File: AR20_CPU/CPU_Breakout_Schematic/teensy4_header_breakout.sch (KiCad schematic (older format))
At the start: 11 parts, among them J3 Micro_SD_Card, SW1 SW_SPST, U1 Teensy_pins, U2 MCP2551-I-SN

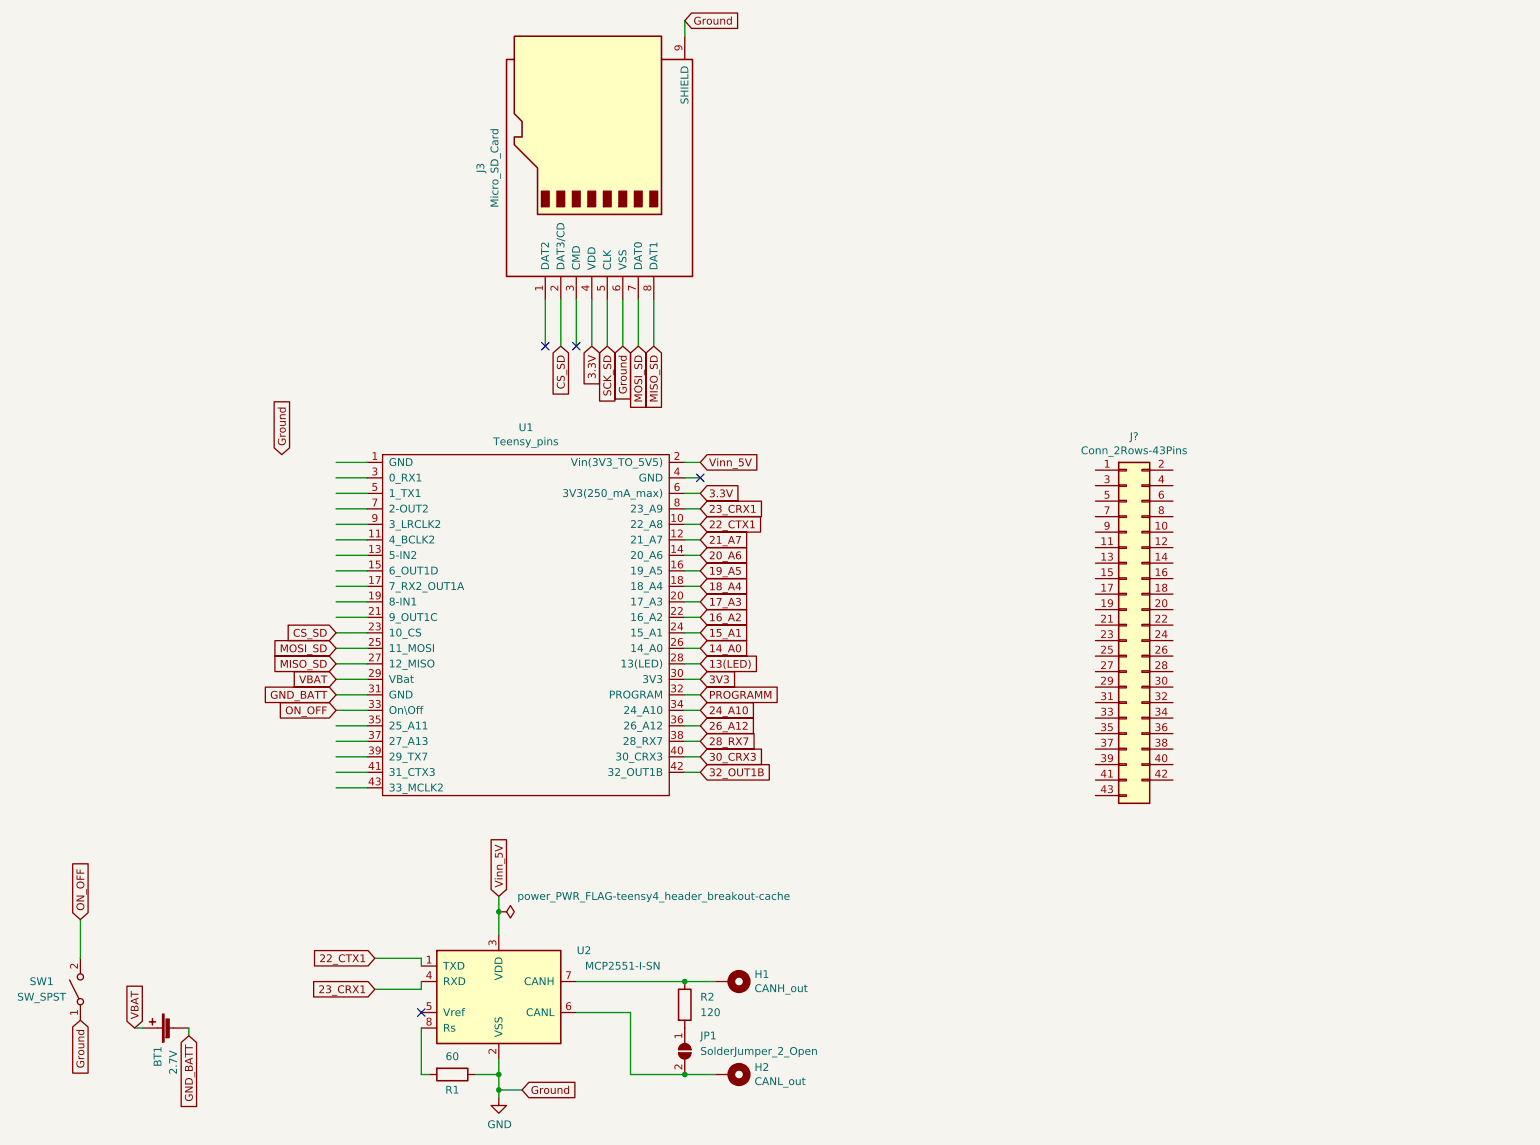
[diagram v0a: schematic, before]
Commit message: FOOTPRINT IS DONE
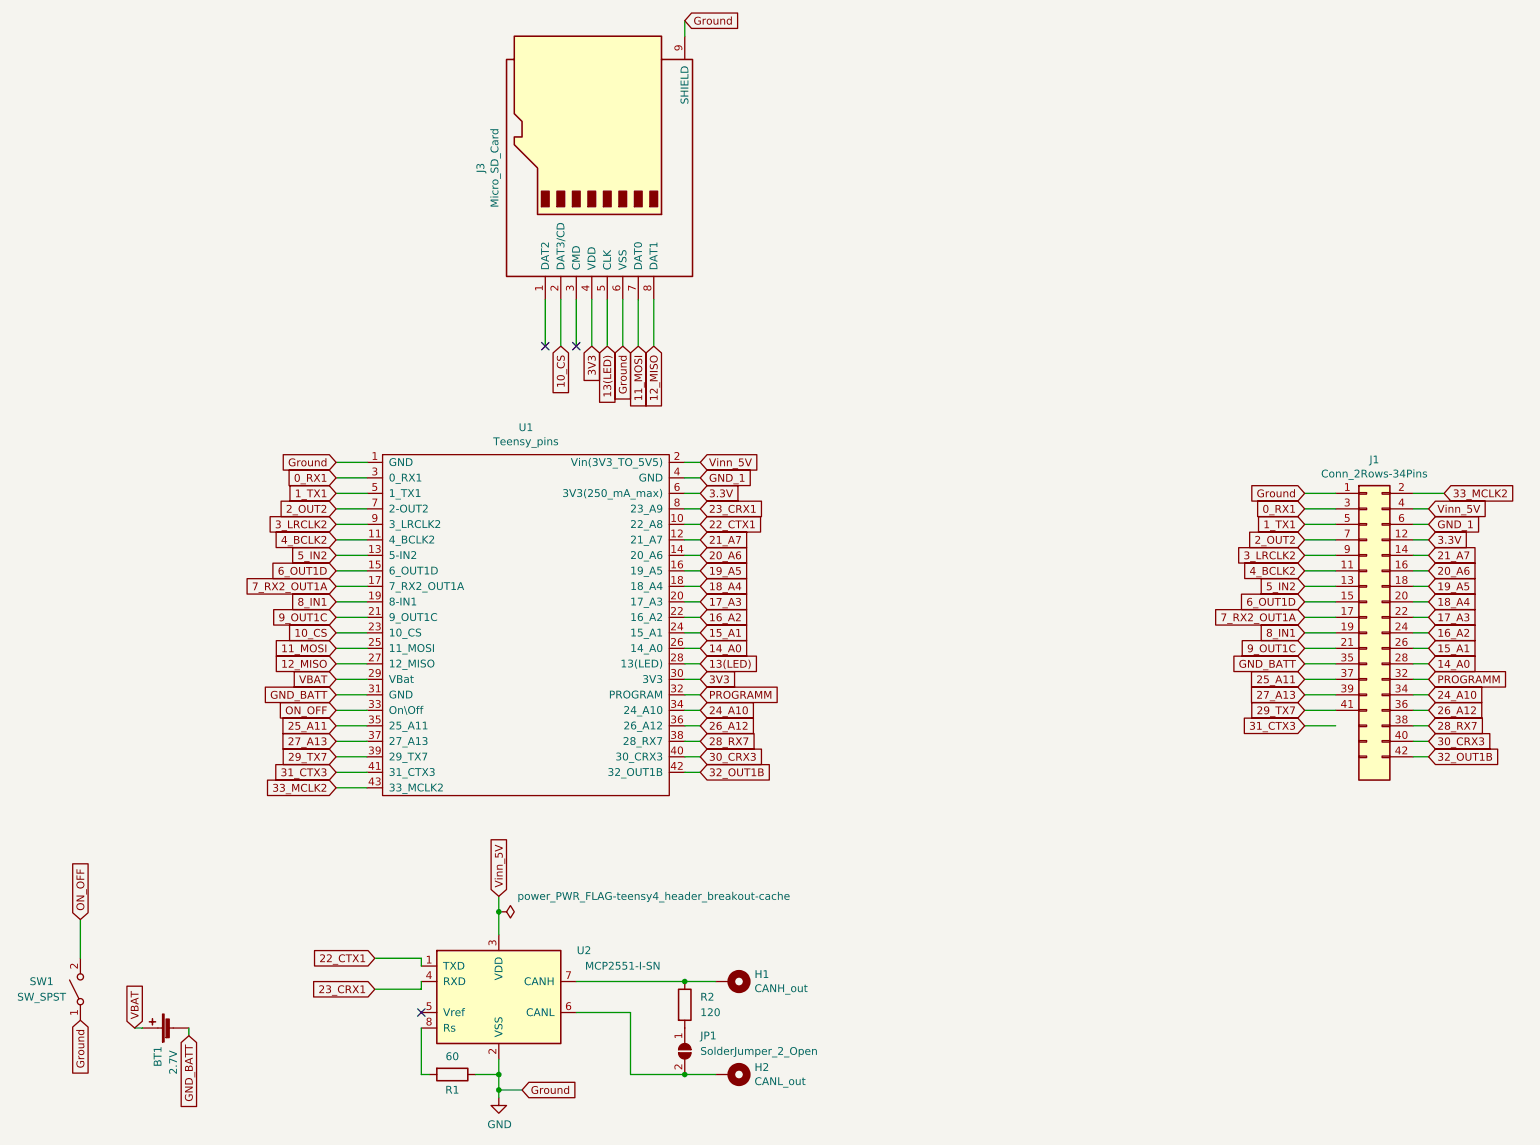
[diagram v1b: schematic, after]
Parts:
- removed J?: Conn_2Rows-43Pins, symbol Connector_Generic:Conn_2Rows-43Pins
- added J1: Conn_2Rows-34Pins, Teensy_Footprint_Library:PINS_IO_TEENSY, symbol BreakoutBoardTeensy:Conn_2Rows-34Pins
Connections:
- net labels added: 0_RX1, 10_CS, 11_MOSI, 12_MISO, 1_TX1, 25_A11, 27_A13, 29_TX7, 2_OUT2, 31_CTX3, 33_MCLK2, 3_LRCLK2, 4_BCLK2, 5_IN2, 6_OUT1D, 7_RX2_OUT1A, 8_IN1, 9_OUT1C, GND_1
- net labels removed: CS_SD, MISO_SD, MOSI_SD, SCK_SD
- wire segments 74 -> 108
- no-connect marks 4 -> 3
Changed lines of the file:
@@
 Text GLabel 2850 6850 0    50   Input ~ 0
 23_CRX1
-Text GLabel 4950 3850 2    50   Input ~ 0
-22_CTX1
-Text GLabel 4950 3750 2    50   Input ~ 0
-23_CRX1
 Text GLabel 3650 6250 1    50   Input ~ 0
 Vinn_5V
-Text GLabel 4950 3450 2    50   Input ~ 0
-Vinn_5V
 $Comp
 L power:GND #PWR0101
@@
 Text GLabel 4450 2700 3    50   Input ~ 0
 Ground
-Text GLabel 2250 3400 1    50   Input ~ 0
+Text GLabel 2600 3450 0    50   Input ~ 0
 Ground
 $Comp
@@
 VBAT
 Text GLabel 2600 4750 0    50   Input ~ 0
-MISO_SD
-Text GLabel 2600 4650 0    50   Input ~ 0
-MOSI_SD
-Text GLabel 2600 4550 0    50   Input ~ 0
-CS_SD
-Text GLabel 4950 4750 2    50   Input ~ 0
-13(LED)
-Text GLabel 4350 2700 3    50   Input ~ 0
-SCK_SD
-Text GLabel 4650 2700 3    50   Input ~ 0
-MISO_SD
-Text GLabel 4550 2700 3    50   Input ~ 0
-MOSI_SD
-Text GLabel 4050 2700 3    50   Input ~ 0
-CS_SD
+12_MISO
 $Bitmap
 Pos 1650 1500
@@
 EndData
 $EndBitmap
-Wire Wire Line
-	4850 3450 4950 3450
-Wire Wire Line
-	4850 3550 4950 3550
-Wire Wire Line
-	4850 3750 4950 3750
-Wire Wire Line
-	4850 3850 4950 3850
 Connection ~ 3650 6350
 Wire Wire Line
@@
 NoConn ~ 3950 2700
 NoConn ~ 4150 2700
-NoConn ~ 4950 3550
 Text GLabel 4850 600  2    50   Input ~ 0
 Ground
 Wire Wire Line
 	4850 700  4850 600
-Text GLabel 4950 3650 2    50   Input ~ 0
-3.3V
-Text GLabel 4250 2700 3    50   Input ~ 0
-3.3V
 Wire Wire Line
 	4250 2400 4250 2700
-$Comp
-L BreakoutBoardTeensy:Teensy_pins U1
-U 1 1 5DD8E484
-P 3250 4150
-F 0 "U1" H 3825 5075 50  0000 C CNN
-F 1 "Teensy_pins" H 3825 4984 50  0000 C CNN
-F 2 "Teensy_Footprint_Library:Teensy_40_footprint" H 4550 4150 50  0001 C CNN
-F 3 "" H 4550 4150 50  0001 C CNN
-	1    3250 4150
-	1    0    0    -1
-$EndComp
 Wire Wire Line
 	2800 4850 2600 4850
@@
 	0    1    1    0
 $EndComp
-$Comp
-L Connector_Generic:Conn_2Rows-43Pins J?
-U 1 1 5DDC3E02
-P 7700 4500
-F 0 "J?" H 7750 5717 50  0000 C CNN
-F 1 "Conn_2Rows-43Pins" H 7750 5626 50  0000 C CNN
-F 2 "" H 7700 4500 50  0001 C CNN
-F 3 "~" H 7700 4500 50  0001 C CNN
-	1    7700 4500
-	1    0    0    -1
-$EndComp
 Wire Wire Line
 	2600 4750 2800 4750
@@
 Wire Wire Line
 	2800 3450 2600 3450
+Text GLabel 2600 3550 0    50   Input ~ 0
+0_RX1
+Text GLabel 2600 3650 0    50   Input ~ 0
+1_TX1
+Text GLabel 2600 3750 0    50   Input ~ 0
+2_OUT2
+Text GLabel 2600 3850 0    50   Input ~ 0
+3_LRCLK2
+Text GLabel 2600 3950 0    50   Input ~ 0
+4_BCLK2
+Text GLabel 2600 4050 0    50   Input ~ 0
+5_IN2
+Text GLabel 2600 4150 0    50   Input ~ 0
+6_OUT1D
+Text GLabel 2600 4250 0    50   Input ~ 0
+7_RX2_OUT1A
+Text GLabel 2600 4350 0    50   Input ~ 0
+8_IN1
+Text GLabel 2600 4450 0    50   Input ~ 0
+9_OUT1C
+Text GLabel 2600 5150 0    50   Input ~ 0
+25_A11
+Text GLabel 2600 5250 0    50   Input ~ 0
+27_A13
+Text GLabel 2600 5350 0    50   Input ~ 0
+29_TX7
+Text GLabel 2600 5450 0    50   Input ~ 0
+31_CTX3
+Text GLabel 2600 5550 0    50   Input ~ 0
+33_MCLK2
+Text GLabel 2600 4550 0    50   Input ~ 0
+10_CS
+Text GLabel 2600 4650 0    50   Input ~ 0
+11_MOSI
+Text GLabel 8850 4750 0    50   Input ~ 0
+GND_BATT
+Text GLabel 8850 3650 0    50   Input ~ 0
+Ground
 Wire Wire Line
-	4850 3950 4950 3950
+	9050 4750 8850 4750
 Wire Wire Line
-	4850 4050 4950 4050
+	9050 4850 8850 4850
 Wire Wire Line
-	4850 4150 4950 4150
+	9050 4950 8850 4950
 Wire Wire Line
-	4850 4250 4950 4250
+	9050 5050 8850 5050
 Wire Wire Line
-	4850 4350 4950 4350
+	9050 5150 8850 5150
 Wire Wire Line
-	4850 4450 4950 4450
+	9550 3650 9750 3650
 Wire Wire Line
-	4850 4550 4950 4550
+	9050 4650 8850 4650
 Wire Wire Line
-	4850 4650 4950 4650
+	9050 4550 8850 4550
 Wire Wire Line
-	4850 4850 4950 4850
+	9050 4450 8850 4450
 Wire Wire Line
-	4850 4950 4950 4950
+	9050 4350 8850 4350
 Wire Wire Line
-	4850 5050 4950 5050
+	9050 4250 8850 4250
 Wire Wire Line
-	4850 5150 4950 5150
+	9050 4150 8850 4150
 Wire Wire Line
-	4850 5250 4950 5250
+	9050 4050 8850 4050
 Wire Wire Line
-	4850 5350 4950 5350
+	9050 3950 8850 3950
 Wire Wire Line
-	4850 5450 4950 5450
+	9050 3850 8850 3850
 Wire Wire Line
-	4950 3650 4850 3650
-Text GLabel 4950 3950 2    50   Input ~ 0
-21_A7
-Text GLabel 4950 4050 2    50   Input ~ 0
-20_A6
-Text GLabel 4950 4150 2    50   Input ~ 0
-19_A5
-Text GLabel 4950 4250 2    50   Input ~ 0
-18_A4
-Text GLabel 4950 4350 2    50   Input ~ 0
-17_A3
-Text GLabel 4950 4450 2    50   Input ~ 0
-16_A2
-Text GLabel 4950 4550 2    50   Input ~ 0
-15_A1
-Text GLabel 4950 4650 2    50   Input ~ 0
-14_A0
-Text GLabel 4950 4850 2    50   Input ~ 0
-3V3
-Text GLabel 4950 4950 2    50   Input ~ 0
-PROGRAMM
-Text GLabel 4950 5050 2    50   Input ~ 0
-24_A10
-Text GLabel 4950 5150 2    50   Input ~ 0
-26_A12
-Text GLabel 4950 5250 2    50   Input ~ 0
-28_RX7
+	9050 3750 8850 3750
+Wire Wire Line
+	9050 3650 8850 3650
+Text GLabel 8850 3750 0    50   Input ~ 0
+0_RX1
+Text GLabel 8850 3850 0    50   Input ~ 0
+1_TX1
+Text GLabel 8850 3950 0    50   Input ~ 0
+2_OUT2
+Text GLabel 8850 4050 0    50   Input ~ 0
+3_LRCLK2
+Text GLabel 8850 4150 0    50   Input ~ 0
+4_BCLK2
+Text GLabel 8850 4250 0    50   Input ~ 0
+5_IN2
+Text GLabel 8850 4350 0    50   Input ~ 0
+6_OUT1D
+Text GLabel 8850 4450 0    50   Input ~ 0
+7_RX2_OUT1A
+Text GLabel 8850 4550 0    50   Input ~ 0
+8_IN1
+Text GLabel 8850 4650 0    50   Input ~ 0
+9_OUT1C
+Text GLabel 8850 4850 0    50   Input ~ 0
+25_A11
+Text GLabel 8850 4950 0    50   Input ~ 0
+27_A13
+Text GLabel 8850 5050 0    50   Input ~ 0
+29_TX7
+Text GLabel 8850 5150 0    50   Input ~ 0
+31_CTX3
+Text GLabel 9750 3650 2    50   Input ~ 0
+33_MCLK2
+Wire Wire Line
+	4950 4750 4850 4750
+Text GLabel 4950 5450 2    50   Input ~ 0
+32_OUT1B
 Text GLabel 4950 5350 2    50   Input ~ 0
 30_CRX3
-Text GLabel 4950 5450 2    50   Input ~ 0
+Text GLabel 4950 5250 2    50   Input ~ 0
+28_RX7
+Text GLabel 4950 5150 2    50   Input ~ 0
+26_A12
+Text GLabel 4950 5050 2    50   Input ~ 0
+24_A10
+Text GLabel 4950 4950 2    50   Input ~ 0
+PROGRAMM
+Text GLabel 4950 4850 2    50   Input ~ 0
+3V3
+Text GLabel 4950 4650 2    50   Input ~ 0
+14_A0
+Text GLabel 4950 4550 2    50   Input ~ 0
+15_A1
+Text GLabel 4950 4450 2    50   Input ~ 0
+16_A2
+Text GLabel 4950 4350 2    50   Input ~ 0
+17_A3
+Text GLabel 4950 4250 2    50   Input ~ 0
+18_A4
+Text GLabel 4950 4150 2    50   Input ~ 0
+19_A5
+Text GLabel 4950 4050 2    50   Input ~ 0
+20_A6
+Text GLabel 4950 3950 2    50   Input ~ 0
+21_A7
+Wire Wire Line
+	4950 3650 4850 3650
+Wire Wire Line
+	4850 5450 4950 5450
+Wire Wire Line
+	4850 5350 4950 5350
+Wire Wire Line
+	4850 5250 4950 5250
+Wire Wire Line
+	4850 5150 4950 5150
+Wire Wire Line
+	4850 5050 4950 5050
+Wire Wire Line
+	4850 4950 4950 4950
+Wire Wire Line
+	4850 4850 4950 4850
+Wire Wire Line
+	4850 4650 4950 4650
+Wire Wire Line
+	4850 4550 4950 4550
+Wire Wire Line
+	4850 4450 4950 4450
+Wire Wire Line
+	4850 4350 4950 4350
+Wire Wire Line
+	4850 4250 4950 4250
+Wire Wire Line
+	4850 4150 4950 4150
+Wire Wire Line
+	4850 4050 4950 4050
+Wire Wire Line
+	4850 3950 4950 3950
+Text GLabel 4950 3650 2    50   Input ~ 0
+3.3V
+Wire Wire Line
+	4850 3850 4950 3850
+Wire Wire Line
+	4850 3750 4950 3750
+Wire Wire Line
+	4850 3550 4950 3550
+Wire Wire Line
+	4850 3450 4950 3450
+Text GLabel 4950 4750 2    50   Input ~ 0
+13(LED)
+Text GLabel 4950 3450 2    50   Input ~ 0
+Vinn_5V
+Text GLabel 4950 3750 2    50   Input ~ 0
+23_CRX1
+Text GLabel 4950 3850 2    50   Input ~ 0
+22_CTX1
+Text GLabel 9650 5350 2    50   Input ~ 0
 32_OUT1B
+Text GLabel 9650 5250 2    50   Input ~ 0
+30_CRX3
+Text GLabel 9650 5150 2    50   Input ~ 0
+28_RX7
+Text GLabel 9650 5050 2    50   Input ~ 0
+26_A12
+Text GLabel 9650 4950 2    50   Input ~ 0
+24_A10
+Text GLabel 9650 4850 2    50   Input ~ 0
+PROGRAMM
+Text GLabel 9650 4750 2    50   Input ~ 0
+14_A0
+Text GLabel 9650 4650 2    50   Input ~ 0
+15_A1
+Text GLabel 9650 4550 2    50   Input ~ 0
+16_A2
+Text GLabel 9650 4450 2    50   Input ~ 0
+17_A3
+Text GLabel 9650 4350 2    50   Input ~ 0
+18_A4
+Text GLabel 9650 4250 2    50   Input ~ 0
+19_A5
+Text GLabel 9650 4150 2    50   Input ~ 0
+20_A6
+Text GLabel 9650 4050 2    50   Input ~ 0
+21_A7
 Wire Wire Line
-	4950 4750 4850 4750
+	9550 5350 9650 5350
+Wire Wire Line
+	9550 5250 9650 5250
+Wire Wire Line
+	9550 5150 9650 5150
+Wire Wire Line
+	9550 5050 9650 5050
+Wire Wire Line
+	9550 4950 9650 4950
+Wire Wire Line
+	9550 4850 9650 4850
+Wire Wire Line
+	9550 4750 9650 4750
+Wire Wire Line
+	9550 4650 9650 4650
+Wire Wire Line
+	9550 4550 9650 4550
+Wire Wire Line
+	9550 4450 9650 4450
+Wire Wire Line
+	9550 4350 9650 4350
+Wire Wire Line
+	9550 4250 9650 4250
+Wire Wire Line
+	9550 4150 9650 4150
+Wire Wire Line
+	9550 4050 9650 4050
+Wire Wire Line
+	9550 3950 9650 3950
+Wire Wire Line
+	9550 3850 9650 3850
+Wire Wire Line
+	9550 3750 9650 3750
+Text GLabel 9650 3750 2    50   Input ~ 0
+Vinn_5V
+Text GLabel 4650 2700 3    50   Input ~ 0
+12_MISO
+Text GLabel 4550 2700 3    50   Input ~ 0
+11_MOSI
+Text GLabel 4050 2700 3    50   Input ~ 0
+10_CS
+Text GLabel 4350 2700 3    50   Input ~ 0
+13(LED)
+Text GLabel 9650 3850 2    50   Input ~ 0
+GND_1
+Text GLabel 4950 3550 2    50   Input ~ 0
+GND_1
+Text GLabel 4250 2700 3    50   Input ~ 0
+3V3
+Text GLabel 9650 3950 2    50   Input ~ 0
+3.3V
+$Comp
+L BreakoutBoardTeensy:Conn_2Rows-34Pins J1
+U 1 1 5DE58733
+P 9250 4550
+F 0 "J1" H 9300 5667 50  0000 C CNN
+F 1 "Conn_2Rows-34Pins" H 9300 5576 50  0000 C CNN
+F 2 "Teensy_Footprint_Library:PINS_IO_TEENSY" H 9250 4550 50  0001 C CNN
+F 3 "~" H 9250 4550 50  0001 C CNN
+	1    9250 4550
+	1    0    0    -1
+$EndComp
+$Comp
+L BreakoutBoardTeensy:Teensy_pins U1
+U 1 1 5DE5DBF9
+P 3250 4150
+F 0 "U1" H 3825 5075 50  0000 C CNN
+F 1 "Teensy_pins" H 3825 4984 50  0000 C CNN
+F 2 "Teensy_Footprint_Library:Teensy_40_footprint" H 4550 4150 50  0001 C CNN
+F 3 "" H 4550 4150 50  0001 C CNN
+	1    3250 4150
+	1    0    0    -1
+$EndComp
 $EndSCHEMATC

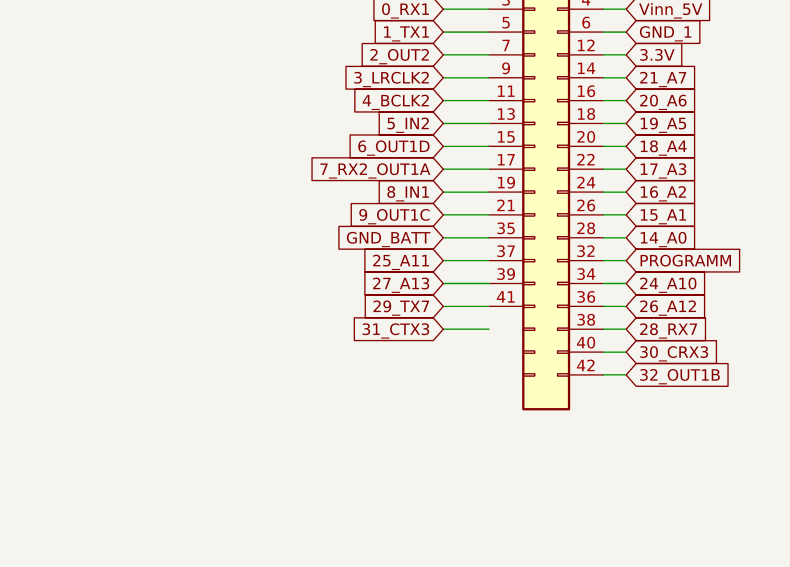
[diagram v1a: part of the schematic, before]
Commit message: initial traces is done
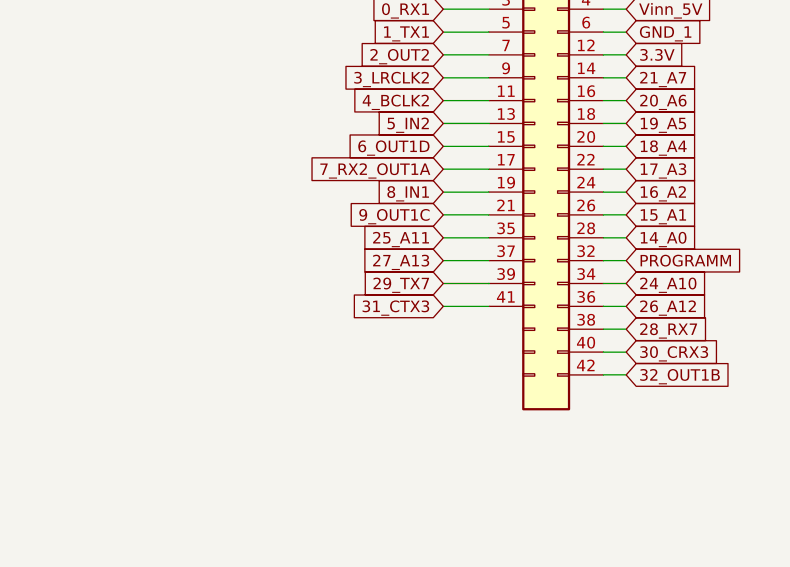
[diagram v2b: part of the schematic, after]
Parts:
- BT1: footprint Battery:BatteryHolder_Keystone_103_1x20mm -> Battery:BatteryHolder_Keystone_3034_1x20mm
- H1, H2: footprint TestPoint:TestPoint_THTPad_D1.0mm_Drill0.5mm -> TestPoint:TestPoint_THTPad_D1.5mm_Drill0.7mm
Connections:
- net 25_A11: now also J1.35 (Pin_35); no longer J1.37 (Pin_37)
- net 27_A13: now also J1.37 (Pin_37); no longer J1.39 (Pin_39)
- net 29_TX7: now also J1.39 (Pin_39); no longer J1.41 (Pin_41)
- net 31_CTX3: now also J1.41 (Pin_41)
- net GND_BATT: no longer J1.35 (Pin_35)
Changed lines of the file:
@@
 F 0 "BT1" H 1300 7200 50  0000 L CNN
 F 1 "2.7V " H 1250 7100 50  0000 L CNN
-F 2 "Battery:BatteryHolder_Keystone_103_1x20mm" V 1550 7160 50  0001 C CNN
+F 2 "Battery:BatteryHolder_Keystone_3034_1x20mm" V 1550 7160 50  0001 C CNN
 F 3 "~" V 1550 7160 50  0001 C CNN
 	1    1550 7100
@@
 F 0 "H2" V 5104 7550 50  0000 L CNN
 F 1 "CANL_out" V 5195 7550 50  0000 L CNN
-F 2 "TestPoint:TestPoint_THTPad_D1.0mm_Drill0.5mm" H 5150 7400 50  0001 C CNN
+F 2 "TestPoint:TestPoint_THTPad_D1.5mm_Drill0.7mm" H 5150 7400 50  0001 C CNN
 F 3 "~" H 5150 7400 50  0001 C CNN
 	1    5150 7400
@@
 F 0 "H1" V 5104 6950 50  0000 L CNN
 F 1 "CANH_out" V 5195 6950 50  0000 L CNN
-F 2 "TestPoint:TestPoint_THTPad_D1.0mm_Drill0.5mm" H 5150 6800 50  0001 C CNN
+F 2 "TestPoint:TestPoint_THTPad_D1.5mm_Drill0.7mm" H 5150 6800 50  0001 C CNN
 F 3 "~" H 5150 6800 50  0001 C CNN
 	1    5150 6800
@@
 Text GLabel 2600 4650 0    50   Input ~ 0
 11_MOSI
-Text GLabel 8850 4750 0    50   Input ~ 0
-GND_BATT
 Text GLabel 8850 3650 0    50   Input ~ 0
 Ground
@@
 	9050 5050 8850 5050
 Wire Wire Line
-	9050 5150 8850 5150
-Wire Wire Line
 	9550 3650 9750 3650
 Wire Wire Line
@@
 Text GLabel 8850 4650 0    50   Input ~ 0
 9_OUT1C
-Text GLabel 8850 4850 0    50   Input ~ 0
+Text GLabel 8850 4750 0    50   Input ~ 0
 25_A11
-Text GLabel 8850 4950 0    50   Input ~ 0
+Text GLabel 8850 4850 0    50   Input ~ 0
 27_A13
-Text GLabel 8850 5050 0    50   Input ~ 0
+Text GLabel 8850 4950 0    50   Input ~ 0
 29_TX7
-Text GLabel 8850 5150 0    50   Input ~ 0
+Text GLabel 8850 5050 0    50   Input ~ 0
 31_CTX3
 Text GLabel 9750 3650 2    50   Input ~ 0
